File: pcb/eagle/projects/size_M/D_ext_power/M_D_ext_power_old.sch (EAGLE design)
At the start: 20 parts

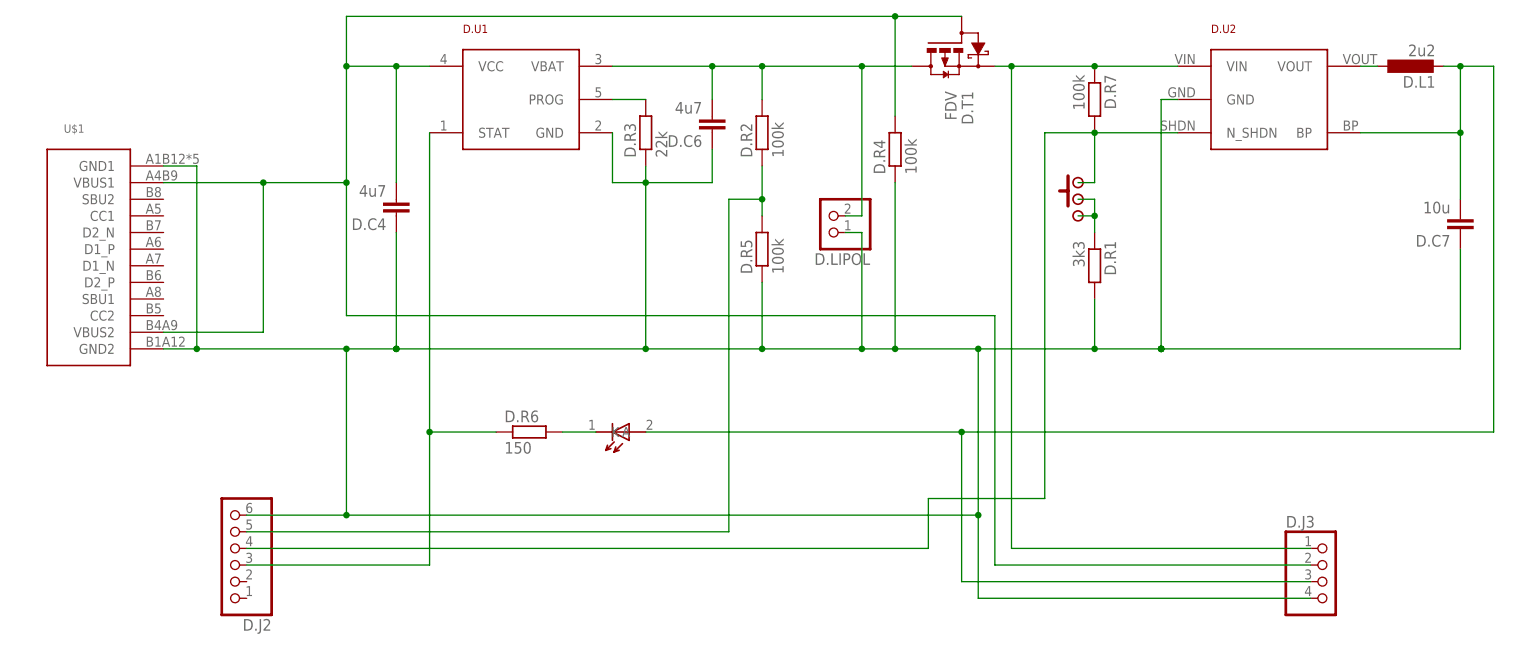
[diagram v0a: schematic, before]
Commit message: PCB M.1
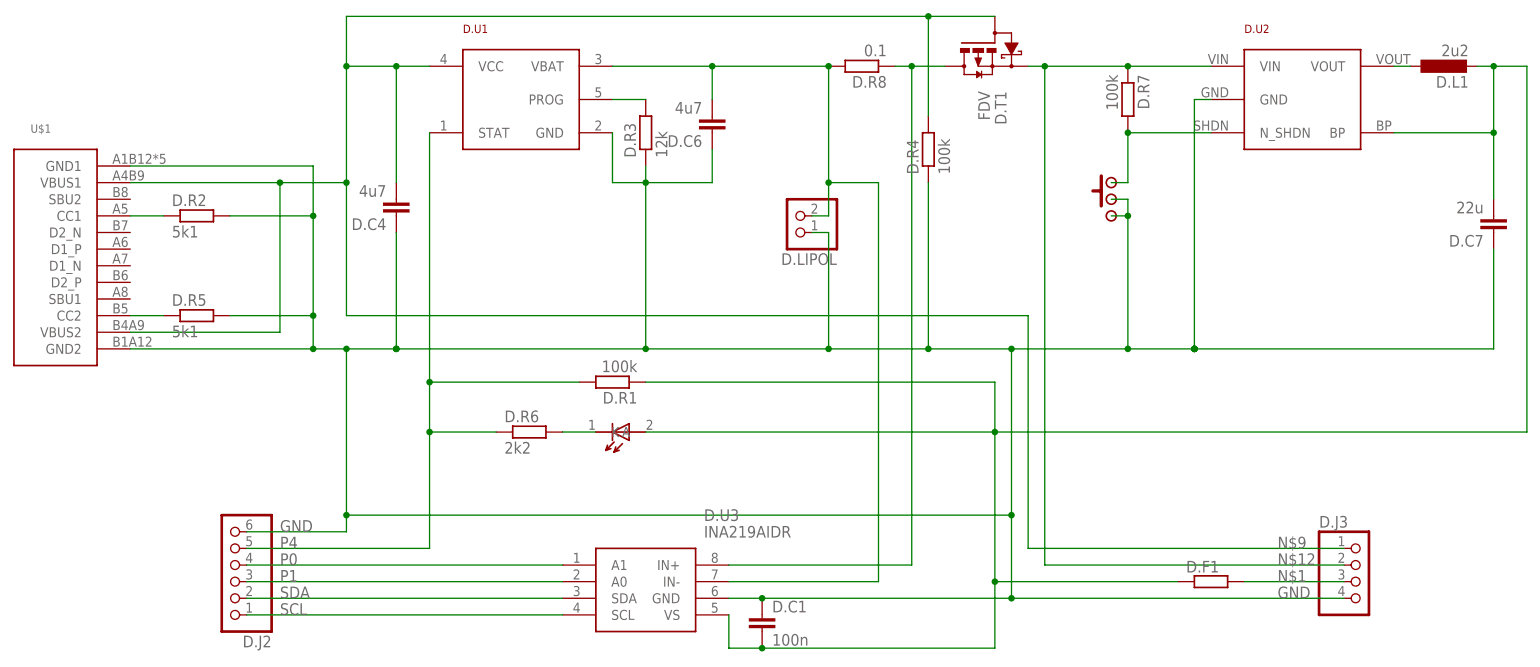
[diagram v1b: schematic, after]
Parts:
- added D.C1: 100n, rcl:C-EUC0603
- added D.F1: (no value), rcl:R-EU_R0805
- added D.R8: 0.1, rcl:R-EU_R0805
- added D.U3: INA219AIDR, SamacSys_Parts:INA219AIDR
- D.C7: value 10u -> 22u; device rcl:C-EUC0603 -> rcl:C-EUC0805
- D.R1: value 3k3 -> 100k
- D.R2, D.R5: value 100k -> 5k1
- D.R3: value 22k -> 12k
- D.R6: value 150 -> 2k2
- D.U2: value TC -> LM3671_3.3
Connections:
- removed net N$20: D.J2.4, D.ON/OFF/RESET.P$1, D.R7.2, D.U2.N_SHDN
- removed net PA7: D.J2.3, D.R6.1, D.U1.STAT
- new net N$13: D.C6.2, D.LIPOL.2, D.R8.2, D.U1.VBAT, D.U3.IN-
- new net N$4: D.R5.1, U$1.CC2
- new net N$6: D.R2.1, U$1.CC1
- new net P0: D.J2.4, D.U3.A1
- new net P1: D.J2.3, D.U3.A0
- new net P4: D.J2.5, D.R1.2, D.R6.1, D.U1.STAT
- new net SCL: D.J2.1, D.U3.SCL
- new net SDA: D.J2.2, D.U3.SDA
- net GND: now also D.C1.1, D.ON/OFF/RESET.P$2, D.ON/OFF/RESET.P$3, D.R2.2, D.R5.2, D.U3.GND; no longer D.R1.2, D.R5.1
- net N$1: now also D.F1.2, D.J3.3; no longer D.ON/OFF/RESET.P$2, D.ON/OFF/RESET.P$3, D.R1.1
- net N$12: now also D.J3.2; no longer D.J3.1
- net N$5: now also D.ON/OFF/RESET.P$1, D.R7.2, D.U2.N_SHDN; no longer D.J2.5, D.R2.1, D.R5.2
- net N$8: now also D.R8.1, D.U3.IN+; no longer D.C6.2, D.LIPOL.2, D.R2.2, D.U1.VBAT
- net N$9: now also D.J3.1; no longer D.J3.2
- net VDD: now also D.C1.2, D.F1.1, D.R1.1, D.U3.VS; no longer D.J3.3
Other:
- moved on the sheet: D.C7, D.J2, D.J3, D.L1, D.LIPOL, D.R1, D.R2, D.R4, D.R5, D.R7, D.T1, D.U2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
